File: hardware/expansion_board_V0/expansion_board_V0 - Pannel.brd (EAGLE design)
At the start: 212 x 132 mm, 499 parts, among them CON1 ELEC, CON10 M5, CON11 M2, CON12 M4, CON13 M1, CON14 ESC0, CON15 CON10_2_2.54, CON16 CON10_2_2.54, CON17 ESC1, CON18 UART0, CON19 QEI1, CON2 SERVO, CON20 AN0, CON21 S0, CON22 IO0, CON23 AN1, CON24 S1, CON25 IO1, CON26 UART1, CON27 QEI0, CON28 AN2, CON29 S2, CON3 LIPO_MOT, CON30 IO2, CON31 TELEM, CON32 QEI3, CON33 AN3, CON34 S3, CON35 IO3, CON36 BALISE, CON37 AN4, CON38 S4, CON39 IO4, CON4 LIPO_MOT, CON40 SPI0, CON41 QEI2, CON42 AN5, CON43 S5, CON44 IO5, CON45 SPI1, CON46 AN6, CON47 S6, CON48 IO6, CON49 I2C0, CON5 LIPO_MOT, CON50 AN7, CON51 S7, CON52 IO7, CON53 I2C1, CON54 USB2, CON55 USB3, CON56 USBfpga, CON57 FPGA_GPIO0, CON58 FPGA_GPIO1, CON59 FPGA_LTC, CON6 LIPO_MOT, CON60 USB3, CON61 CON5_2.54S, CON62 CON5_2.54S, CON63 CON5_2.54S, CON64 CON5_2.54S, CON7 FPGApower, CON8 M0, CON9 M3, IC1 ADS1258, IC2 ADS1278, IC3 REF5030I, IC4 REF5025I, J1 NC, J10 0, J11 0, J12 0, J13 0, J14 0, J15 0, J16 0, J17 0, J18 0, J19 0, J2 nc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

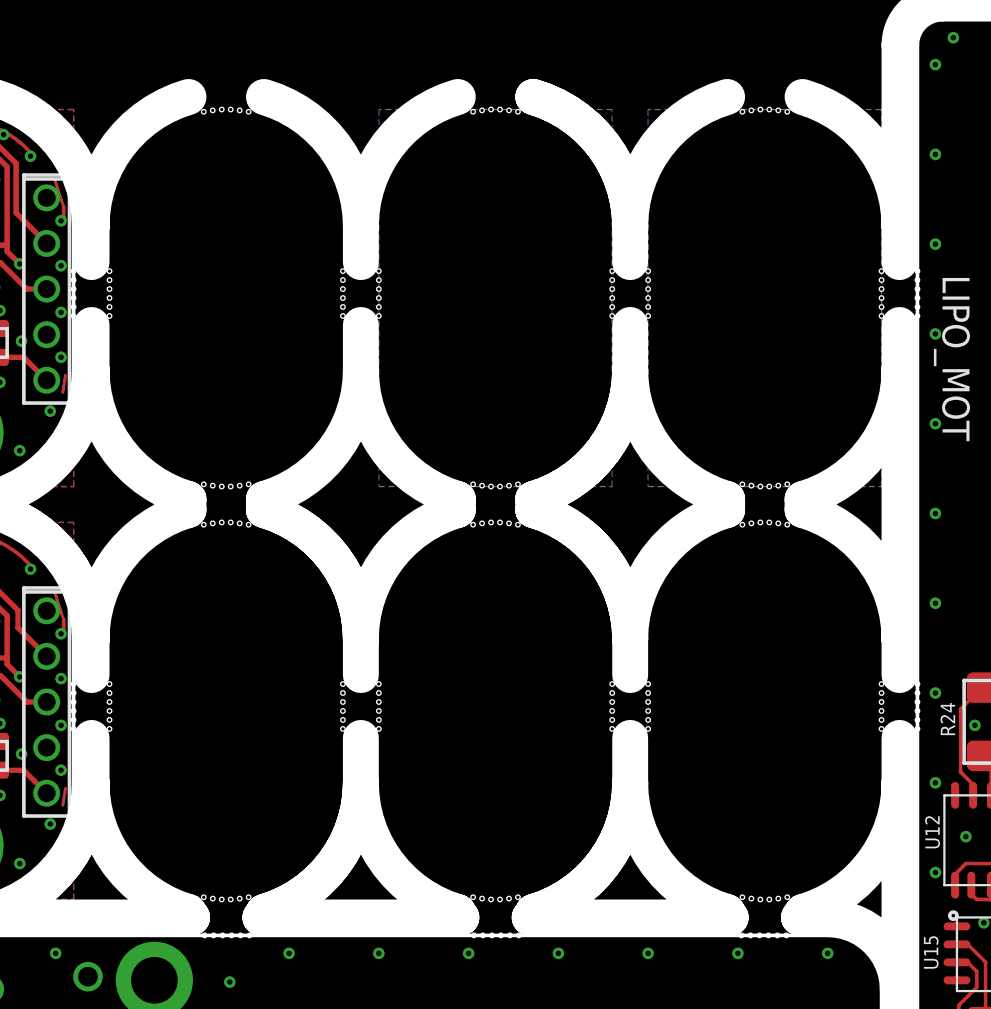
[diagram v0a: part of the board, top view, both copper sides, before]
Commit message: -
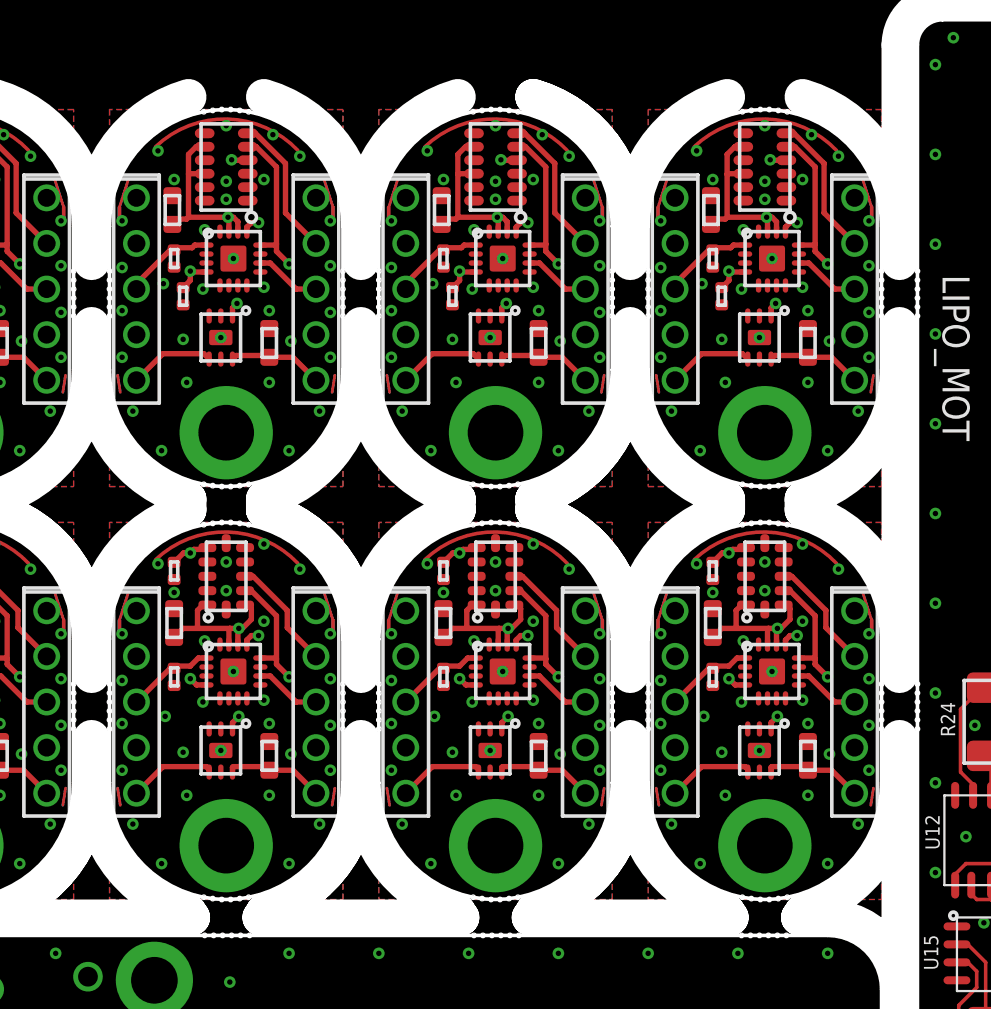
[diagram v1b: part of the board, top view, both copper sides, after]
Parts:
- added C200, C201, C202, C203, C204, C205, C206, C207, C208, C209, C210, C211: 2u, iocene:CAPC1608X95N
- added CON65, CON66, CON67, CON68, CON69, CON70, CON71, CON72, CON73, CON74, CON75, CON76: CON5_2.54S, iocene:CON254P1270X400-5S
- added R111, R112, R113, R114, R115, R116, R117, R118, R119, R120, R121, R122: 10k, iocene:RESC1005X40N
- added U41, U47, U53: VL53L0X, iocene:VL53L0X
- added U42, U44, U48, U50, U54, U56: TCA6408A, iocene:QFN50P300X300X80-17N
- added U43, U45, U49, U51, U55, U57: LP5900SD-2.8, iocene:SON65P250X220X80-7N
- added U46, U52, U58: VL6180X, iocene:VL6180X
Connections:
- new net GND1: C200.P$2, C201.P$2, C202.P$2, C203.P$2, CON65.1, CON66.1, CON67.1, CON68.1, R111.2, R112.2, R113.2, R114.2, U41.P$12, U41.P$2, U41.P$3, U41.P$4, U41.P$6, U42.GND, U42.P$16, U42.P$6, U43.2, U43.3, U43.5, U43.GND, U44.GND, U44.P$16, U44.P$6, U45.2, U45.3, U45.5, U45.GND, U46.P$11, U46.P$12, U46.P$2, U46.P$3, U46.P$7, U46.P$9
- new net GND2: C204.P$2, C205.P$2, C206.P$2, C207.P$2, CON69.1, CON70.1, CON71.1, CON72.1, R115.2, R116.2, R117.2, R118.2, U47.P$12, U47.P$2, U47.P$3, U47.P$4, U47.P$6, U48.GND, U48.P$16, U48.P$6, U49.2, U49.3, U49.5, U49.GND, U50.GND, U50.P$16, U50.P$6, U51.2, U51.3, U51.5, U51.GND, U52.P$11, U52.P$12, U52.P$2, U52.P$3, U52.P$7, U52.P$9
- new net GND3: C208.P$2, C209.P$2, C210.P$2, C211.P$2, CON73.1, CON74.1, CON75.1, CON76.1, R119.2, R120.2, R121.2, R122.2, U53.P$12, U53.P$2, U53.P$3, U53.P$4, U53.P$6, U54.GND, U54.P$16, U54.P$6, U55.2, U55.3, U55.5, U55.GND, U56.GND, U56.P$16, U56.P$6, U57.2, U57.3, U57.5, U57.GND, U58.P$11, U58.P$12, U58.P$2, U58.P$3, U58.P$7, U58.P$9
- new net N$107: CON66.3, R112.1, U42.P$1
- new net N$108: CON65.2, CON66.2, U41.P$9, U42.P$13
- new net N$109: CON65.4, CON66.4, U41.P$10, U42.P$12
- new net N$122: CON65.3, U42.P$10
- new net N$137: C201.P$1, CON65.5, CON66.5, U43.4, U43.6
- new net N$140: C200.P$1, U41.P$1, U41.P$11, U42.P$14, U42.P$15, U43.1
- new net N$141: C203.P$1, CON67.5, CON68.5, U45.4, U45.6
- new net N$142: CON67.4, CON68.4, U44.P$12, U46.P$5
- new net N$143: CON67.2, CON68.2, U44.P$13, U46.P$6
- new net N$144: C202.P$1, U44.P$14, U44.P$15, U45.1, U46.P$10, U46.P$8
- new net N$145: CON68.3, R114.1, U44.P$1
- new net N$146: CON67.3, U44.P$10
- new net N$147: R113.1, U44.P$4, U46.P$4
- new net N$148: R115.1, U47.P$5, U48.P$4
- new net N$152: CON70.3, R116.1, U48.P$1
- new net N$165: CON69.2, CON70.2, U47.P$9, U48.P$13
- new net N$179: CON69.4, CON70.4, U47.P$10, U48.P$12
- new net N$183: CON69.3, U48.P$10
- new net N$186: C205.P$1, CON69.5, CON70.5, U49.4, U49.6
- new net N$194: C204.P$1, U47.P$1, U47.P$11, U48.P$14, U48.P$15, U49.1
- new net N$197: C207.P$1, CON71.5, CON72.5, U51.4, U51.6
- new net N$203: CON71.4, CON72.4, U50.P$12, U52.P$5
- new net N$209: CON71.2, CON72.2, U50.P$13, U52.P$6
- new net N$215: C206.P$1, U50.P$14, U50.P$15, U51.1, U52.P$10, U52.P$8
- new net N$216: CON72.3, R118.1, U50.P$1
- new net N$217: CON71.3, U50.P$10
- new net N$218: R117.1, U50.P$4, U52.P$4
- new net N$222: R119.1, U53.P$5, U54.P$4
- new net N$226: CON74.3, R120.1, U54.P$1
- new net N$227: CON73.2, CON74.2, U53.P$9, U54.P$13
- new net N$228: CON73.4, CON74.4, U53.P$10, U54.P$12
- new net N$229: CON73.3, U54.P$10
- new net N$230: C209.P$1, CON73.5, CON74.5, U55.4, U55.6
- new net N$231: C208.P$1, U53.P$1, U53.P$11, U54.P$14, U54.P$15, U55.1
- new net N$233: C211.P$1, CON75.5, CON76.5, U57.4, U57.6
- new net N$234: CON75.4, CON76.4, U56.P$12, U58.P$5
- new net N$235: CON75.2, CON76.2, U56.P$13, U58.P$6
- new net N$236: C210.P$1, U56.P$14, U56.P$15, U57.1, U58.P$10, U58.P$8
- new net N$237: CON76.3, R122.1, U56.P$1
- new net N$238: CON75.3, U56.P$10
- new net N$239: R121.1, U56.P$4, U58.P$4
- new net N$98: R111.1, U41.P$5, U42.P$4
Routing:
- net GND3: track 0.00 -> 70.3 mm, vias 0 -> 63
- net GND2: track 0.00 -> 70.3 mm, vias 0 -> 63
- net GND1: track 0.00 -> 70.3 mm, vias 0 -> 63
- net N$234: track 0.00 -> 22.5 mm, vias 0 -> 1
- net N$203: track 0.00 -> 22.5 mm, vias 0 -> 1
- net N$142: track 0.00 -> 22.5 mm, vias 0 -> 1
- net N$230: track 0.00 -> 21.2 mm
- net N$186: track 0.00 -> 21.2 mm
- net N$137: track 0.00 -> 21.2 mm
- net N$233: track 0.00 -> 21.0 mm
- net N$197: track 0.00 -> 21.0 mm
- net N$141: track 0.00 -> 21.0 mm
- net N$228: track 0.00 -> 20.8 mm, vias 0 -> 1
- net N$179: track 0.00 -> 20.8 mm, vias 0 -> 1
- net N$109: track 0.00 -> 20.8 mm, vias 0 -> 1
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- added copper zone on layer 1, net GND1
- added copper zone on layer 15, net GND1
- added copper zone on layer 16, net GND1
- added copper zone on layer 2, net GND1
- added copper zone on layer 1, net GND2
- added copper zone on layer 15, net GND2
- added copper zone on layer 16, net GND2
- added copper zone on layer 2, net GND2
- added copper zone on layer 1, net GND3
- added copper zone on layer 15, net GND3
- added copper zone on layer 16, net GND3
- added copper zone on layer 2, net GND3
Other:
- outline, holes or cut-outs redrawn
